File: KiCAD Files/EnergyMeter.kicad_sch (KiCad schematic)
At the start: 56 parts, among them J1 Screw_Terminal_AC, J2 Conn_01x05, J3 Screw_Terminal_LOAD, Q1 BSS138, Q2 BSS138, Q3 S8050-SOT23, Q4 S8050-SOT23, SW1 SW_Push, U1 AMS1117-3.3, U2 ESP-12F, U3 HLW8032

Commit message: V1rev1
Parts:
- H1, H2, H3, H4: footprint MountingHole:MountingHole_3.2mm_M3 -> MountingHole:MountingHole_3.2mm_M3_Pad_TopBottom
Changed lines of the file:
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@@
 			)
 		)
-		(property "Footprint" "MountingHole:MountingHole_3.2mm_M3"
+		(property "Footprint" "MountingHole:MountingHole_3.2mm_M3_Pad_TopBottom"
 			(at 99.06 185.42 0)
 			(effects
@@
 			)
 		)
-		(property "Footprint" "MountingHole:MountingHole_3.2mm_M3"
+		(property "Footprint" "MountingHole:MountingHole_3.2mm_M3_Pad_TopBottom"
 			(at 137.16 185.42 0)
 			(effects
@@
 			)
 		)
-		(property "Footprint" "MountingHole:MountingHole_3.2mm_M3"
+		(property "Footprint" "MountingHole:MountingHole_3.2mm_M3_Pad_TopBottom"
 			(at 118.11 185.42 0)
 			(effects
@@
 			)
 		)
-		(property "Footprint" "MountingHole:MountingHole_3.2mm_M3"
+		(property "Footprint" "MountingHole:MountingHole_3.2mm_M3_Pad_TopBottom"
 			(at 80.01 185.42 0)
 			(effects

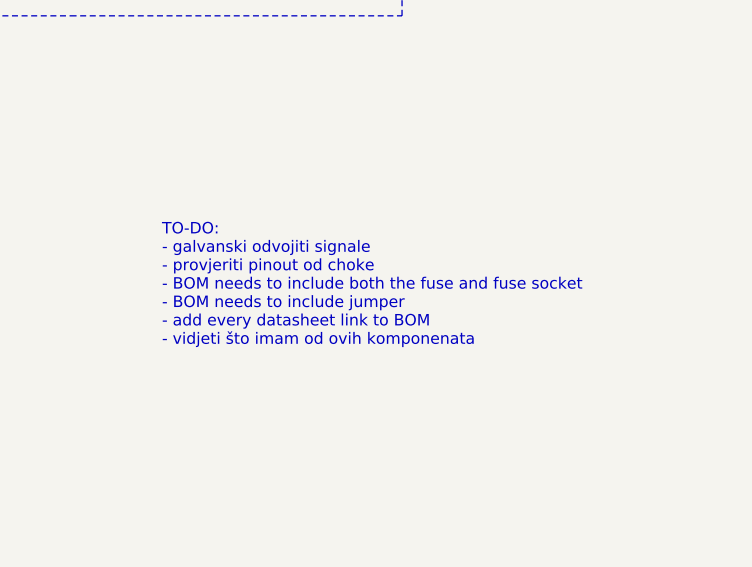
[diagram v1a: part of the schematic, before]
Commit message: update
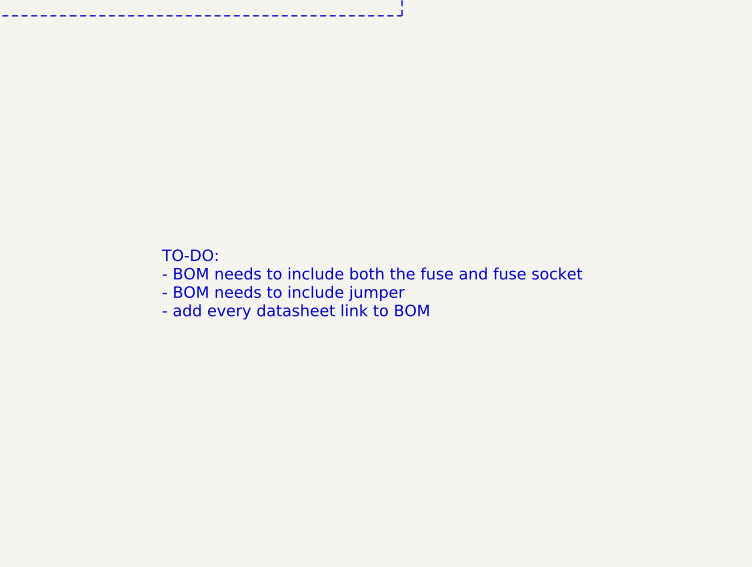
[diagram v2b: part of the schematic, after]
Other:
- note added: "TO-DO: - BOM needs to include both the fuse and fuse socket - BOM needs to include jumper - add every datasheet link to BOM"
- note removed: "TO-DO: - galvanski odvojiti signale - provjeriti pinout od choke - BOM needs to include both the fuse and fuse socket - BOM needs to include jumper - add every datasheet link to BOM - vidjeti što imam od ovih komponenata"
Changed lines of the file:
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@@
 		)
 	)
-	(text "TO-DO:\n- galvanski odvojiti signale\n- provjeriti pinout od choke\n- BOM needs to include both the fuse and fuse socket\n- BOM needs to include jumper\n- add every datasheet link to BOM\n- vidjeti što imam od ovih komponenata\n"
+	(text "TO-DO:\n- BOM needs to include both the fuse and fuse socket\n- BOM needs to include jumper\n- add every datasheet link to BOM\n"
 		(exclude_from_sim no)
 		(at 227.33 153.162 0)
